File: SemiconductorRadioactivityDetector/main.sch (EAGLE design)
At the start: 27 parts, among them IC1 4011D, J1 22-05-7028-02, J2 22-05-7028-02, J3 22-05-7028-02, Q1 IRF530

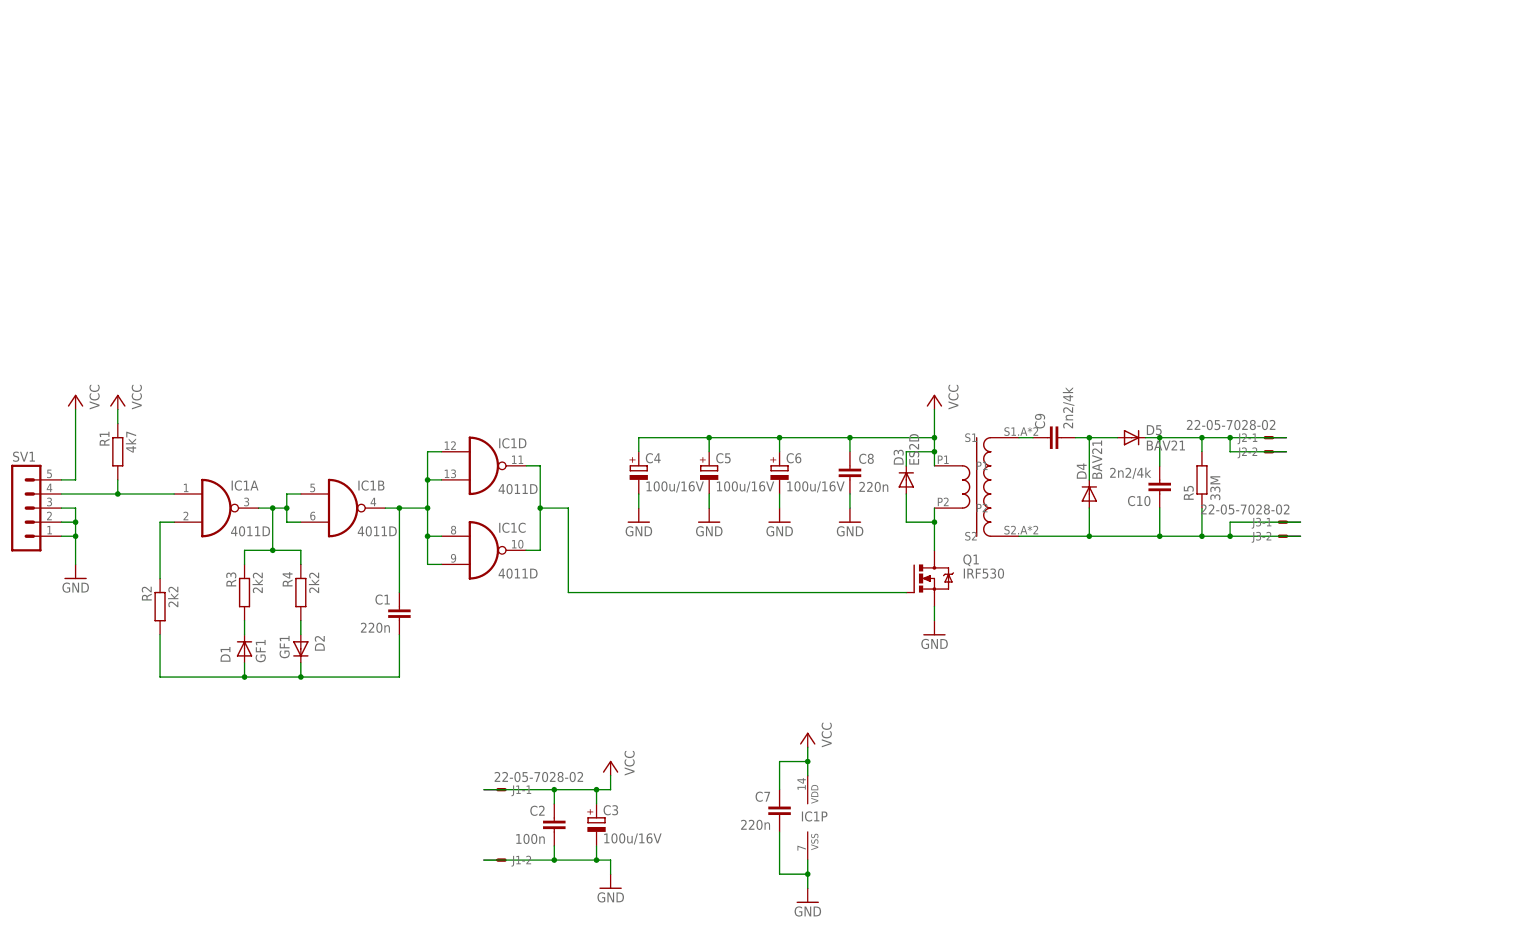
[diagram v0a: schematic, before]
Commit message: Initial unfinished version.
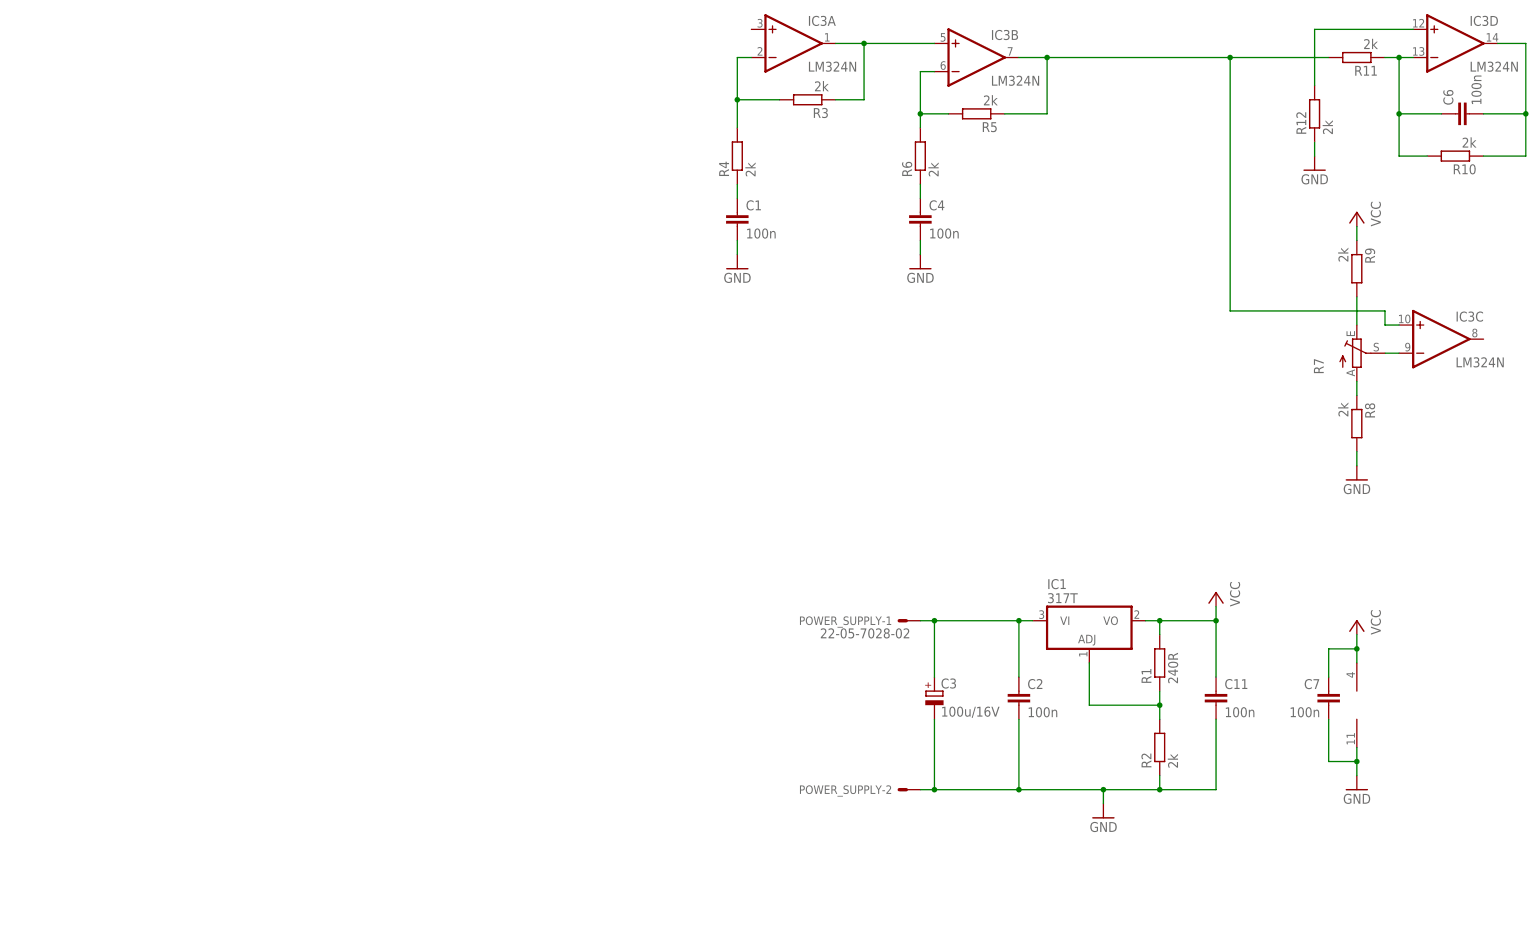
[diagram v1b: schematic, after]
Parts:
- removed 11: CCFL_INVERTER_COIL, ccfl_inverter_coil:CCFL_INVERTER_COIL
- removed C10: 2n2/4k, resistor:C-EU075-042X103
- removed C5: 100u/16V, resistor:CPOL-EU153CLV-0505
- removed C8: 220n, resistor:C-EUC0805
- removed C9: 2n2/4k, rcl:C-EU075-042X103
- removed D1, D2: GF1, diode:GF1
- removed D3: ES2D, diode:ES2D
- removed D4, D5: BAV21, diode:BAV21
- removed J1, J2, J3: 22-05-7028-02, con-molex:22-05-7028-02
- removed Q1: IRF530, transistor-power:IRF530
- removed SV1: (no value), con-lstb:MA05-1
- added C11: 100n, resistor:C-EUC1206
- added IC3: LM324N, linear:LM324N
- added POWER_SUPPLY: 22-05-7028-02, con-molex:22-05-7028-02
- added R10, R11, R12, R6, R8, R9: 2k, resistor:R-EU_M1206
- added R7: (no value), pot:TRIM_EU-B64Y
- C1: value 220n -> 100n; device resistor:C-EU025-025X050 -> resistor:C-EUC1206
- C2: device resistor:C-EUC0805 -> resistor:C-EUC1206
- C4, C6: value 100u/16V -> 100n; device rcl:CPOL-EU153CLV-0505 -> resistor:C-EUC1206
- C7: value 220n -> 100n; device resistor:C-EUC0805 -> resistor:C-EUC1206
- IC1: value 4011D -> 317T; device 40xx:4011D -> linear:317T
- R1: value 4k7 -> 240R; device resistor:R-EU_M0805 -> resistor:R-EU_M1206
- R2, R3, R4: value 2k2 -> 2k; device resistor:R-EU_M0805 -> resistor:R-EU_M1206
- R5: value 33M -> 2k; device resistor:R-EU_0207/10 -> resistor:R-EU_M1206
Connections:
- removed net N$22: IC1A.O, IC1B.I0, IC1B.I1, R3.1, R4.1
- removed net N$23: C1.2, D1.A, D2.C, R2.2
- removed net N$24: D1.C, R3.2
- removed net N$25: D2.A, R4.2
- new net N$12: C6.1, IC3D.-IN, R10.2, R11.1
- new net N$13: C6.2, IC3D.OUT, R10.1
- new net N$14: IC3D.+IN, R12.2
- new net N$8: C2.1, C3.+, IC1.VI, POWER_SUPPLY-1.S
- new net N$9: R7.E, R9.2
- net GND: now also C1.2, C11.2, C4.2, IC3P.V-, POWER_SUPPLY-2.S, R12.1, R2.1, R8.2; no longer C4.-, C5.-, C6.-, C8.2, IC1P.VSS, J1-2.S, Q1.S, SV1.1, SV1.2, SV1.3
- net N$1: now also IC1.ADJ, R1.1, R2.2; no longer IC1A.I1, R2.1
- net N$10: now also R7.A, R8.1; no longer C10.2, D5.C, J2-1.S, J2-2.S, R5.2
- net N$11: now also IC3C.-IN, R7.S; no longer 11.S2, C10.1, D4.A, J3-1.S, J3-2.S, R5.1
- net N$2: now also IC3A.-IN, R3.2, R4.2; no longer IC1A.I0, R1.2, SV1.4
- net N$3: now also IC3A.OUT, IC3B.+IN, R3.1; no longer 11.P2, D3.A, Q1.D
- net N$4: now also C1.1, R4.1; no longer IC1C.O, IC1D.O, Q1.G
- net N$5: now also IC3B.-IN, R5.2, R6.2; no longer C1.1, IC1B.O, IC1C.I0, IC1C.I1, IC1D.I0, IC1D.I1
- net N$6: now also IC3B.OUT, IC3C.+IN, R11.2, R5.1; no longer 11.S1, C9.1
- net N$7: now also C4.1, R6.1; no longer C9.2, D4.C, D5.A
- net VCC: now also C11.1, IC1.VO, IC3P.V+, R1.2, R9.1; no longer 11.P1, C2.1, C3.+, C4.+, C5.+, C6.+, C8.1, D3.C, IC1P.VDD, J1-1.S, R1.1, SV1.5
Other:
- moved on the sheet: C1, C2, C3, C7, R1, R2, R3, R4, R5
